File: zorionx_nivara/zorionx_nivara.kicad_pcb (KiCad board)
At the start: 4 copper layers, 102.2 x 83 mm, 29 parts, among them J1 Screw_Terminal_3_P5.00mm, J12 Screw_Terminal_4_P5.00mm, J13 Screw_Terminal_6_P5.00mm, J14 Screw_Terminal_2_P5.00mm, J2 Screw_Terminal_2_P5.00mm, J3 Screw_Terminal_2_P5.00mm, J4 Screw_Terminal_4_P5.00mm, J5 Screw_Terminal_2_P5.00mm, J6 Screw_Terminal_2_P5.00mm, J9 Screw_Terminal_3_P5.00mm, U1 ESP32-S3-WROOM-1, U2 AP63203WU

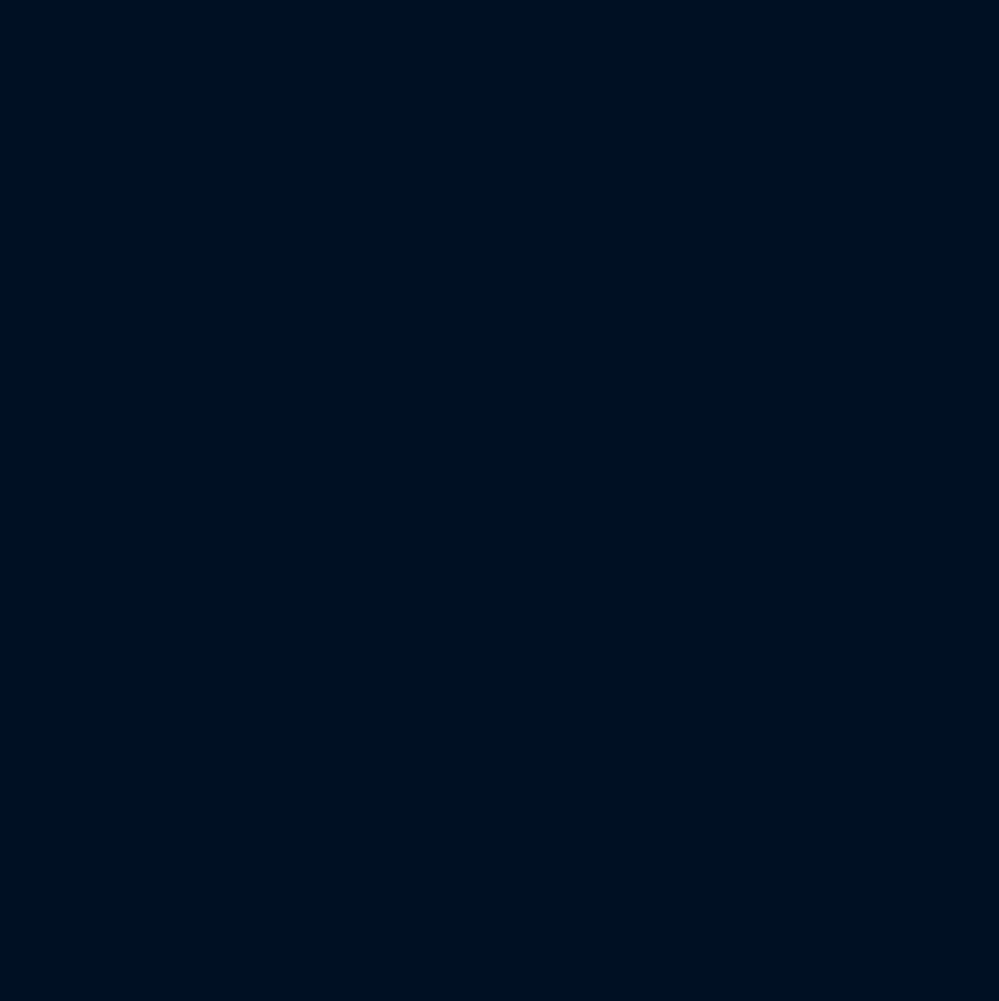
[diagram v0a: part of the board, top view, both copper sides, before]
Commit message: Salvado
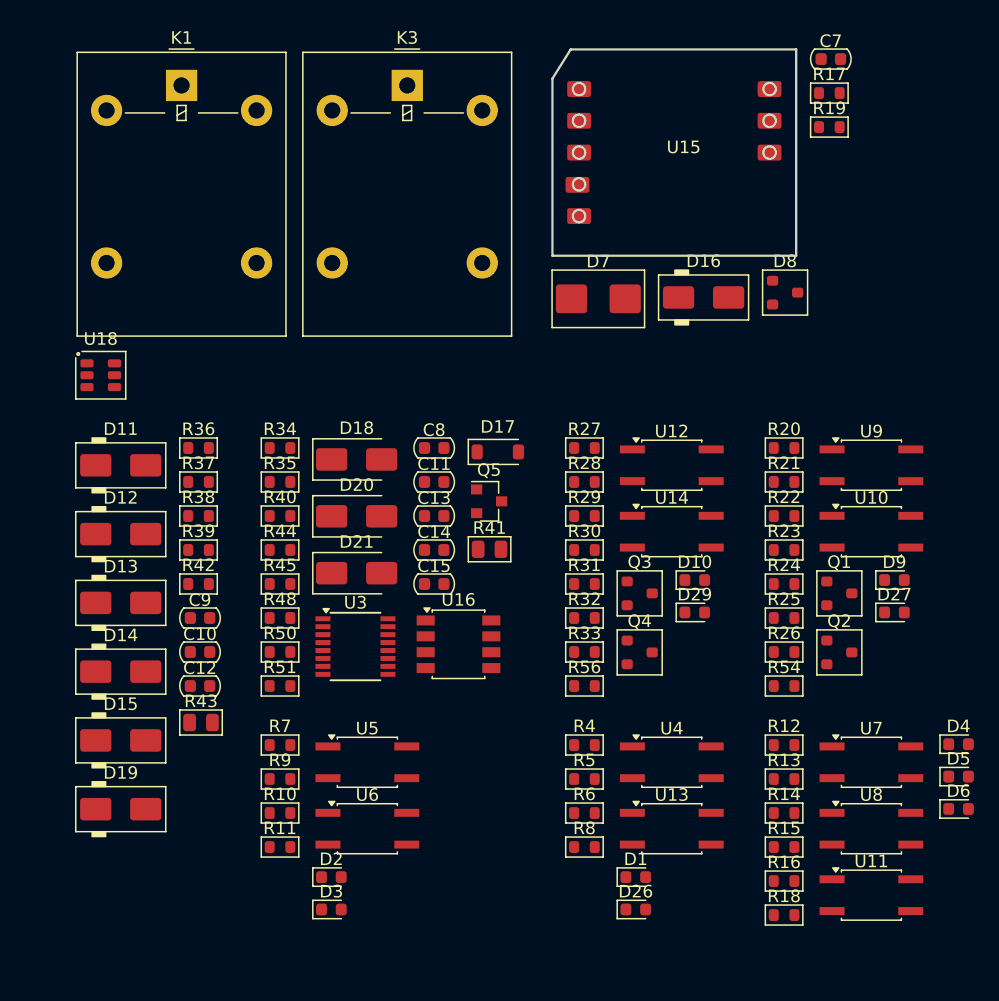
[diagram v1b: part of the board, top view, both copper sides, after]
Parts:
- added C10: 100nF, PCM_Capacitor_SMD_AKL:C_0603_1608Metric, F.Cu at (219.6, 65.1)
- added C11: 0.1uF, PCM_Capacitor_SMD_AKL:C_0603_1608Metric, F.Cu at (238.3, 51.5)
- added C12: 100nF, PCM_Capacitor_SMD_AKL:C_0603_1608Metric, F.Cu at (219.6, 67.9)
- added C13: 220pF, PCM_Capacitor_SMD_AKL:C_0603_1608Metric, F.Cu at (238.3, 54.3)
- added C14: 1uF, PCM_Capacitor_SMD_AKL:C_0603_1608Metric, F.Cu at (238.3, 57.0)
- added C15: 0.1uF, PCM_Capacitor_SMD_AKL:C_0603_1608Metric, F.Cu at (238.3, 59.7)
- added C7: 10uF, PCM_Capacitor_SMD_AKL:C_0603_1608Metric, F.Cu at (270.0, 17.7)
- added C8: 1uF, PCM_Capacitor_SMD_AKL:C_0603_1608Metric, F.Cu at (238.3, 48.8)
- added C9: 100nF, PCM_Capacitor_SMD_AKL:C_0603_1608Metric, F.Cu at (219.6, 62.4)
- added D1: LED ON, LED_SMD:LED_0603_1608Metric, F.Cu at (254.4, 83.1)
- added D10: LED ON, LED_SMD:LED_0603_1608Metric, F.Cu at (259.2, 59.4)
- added D11: SMAJ5.0A, PCM_Diode_SMD_AKL:D_SMA, F.Cu at (213.2, 50.2)
- added D12: SMAJ5.0A, PCM_Diode_SMD_AKL:D_SMA, F.Cu at (213.2, 55.7)
- added D13: SMAJ5.0A, PCM_Diode_SMD_AKL:D_SMA, F.Cu at (213.2, 61.2)
- added D14: SMAJ5.0A, PCM_Diode_SMD_AKL:D_SMA, F.Cu at (213.2, 66.7)
- added D15: SMAJ5.0A, PCM_Diode_SMD_AKL:D_SMA, F.Cu at (213.2, 72.2)
- added D16: SMAJ5.0A, PCM_Diode_SMD_AKL:D_SMA, F.Cu at (259.9, 36.8)
- added D17: BZT52C12_C2891780, Diode_SMD:D_SOD-123, F.Cu at (243.4, 49.1)
- added D18: SMAJ12A, Diode_SMD:D_SMA, F.Cu at (232.1, 49.7)
- added D19: SMAJ5.0A, PCM_Diode_SMD_AKL:D_SMA, F.Cu at (213.2, 77.7)
- added D2: LED ON, LED_SMD:LED_0603_1608Metric, F.Cu at (230.1, 83.1)
- added D20: SMAJ33A, Diode_SMD:D_SMA, F.Cu at (232.1, 54.3)
- added D21: MRA4007T3G, Diode_SMD:D_SMA, F.Cu at (232.1, 58.8)
- added D26: LED ON, LED_SMD:LED_0603_1608Metric, F.Cu at (254.4, 85.7)
- added D27: LED ON, LED_SMD:LED_0603_1608Metric, F.Cu at (275.1, 62.0)
- added D29: LED ON, LED_SMD:LED_0603_1608Metric, F.Cu at (259.2, 62.0)
- added D3: LED ON, LED_SMD:LED_0603_1608Metric, F.Cu at (230.1, 85.7)
- added D4: LED ON, LED_SMD:LED_0603_1608Metric, F.Cu at (280.3, 72.5)
- added D5: LED ON, LED_SMD:LED_0603_1608Metric, F.Cu at (280.3, 75.1)
- added D6: LED ON, LED_SMD:LED_0603_1608Metric, F.Cu at (280.3, 77.7)
- added D7: SMBJ12CA, PCM_Diode_SMD_AKL:D_SMB_TVS, F.Cu at (251.4, 36.9)
- added D8: SM712, PCM_Package_TO_SOT_SMD_AKL:SOT-23, F.Cu at (266.4, 36.4)
- added D9: LED ON, LED_SMD:LED_0603_1608Metric, F.Cu at (275.1, 59.4)
- added K1: G5LE-1, Relay_THT:Relay_SPDT_Omron-G5LE-1, F.Cu at (218.1, 19.8)
- added K3: G5LE-1, Relay_THT:Relay_SPDT_Omron-G5LE-1, F.Cu at (236.2, 19.8)
- added Q1: AO3407A, PCM_Package_TO_SOT_SMD_AKL:SOT-23, F.Cu at (270.7, 60.5)
- added Q2: AO3407A, PCM_Package_TO_SOT_SMD_AKL:SOT-23, F.Cu at (270.7, 65.2)
- added Q3: IRLML0040, PCM_Package_TO_SOT_SMD_AKL:SOT-23, F.Cu at (254.7, 60.5)
- added Q4: IRLML0040, PCM_Package_TO_SOT_SMD_AKL:SOT-23, F.Cu at (254.7, 65.2)
- added Q5: IRLML6402TRPBF-JSM, PCM_4ms_Package_SOT:SOT-23, F.Cu at (242.7, 53.1)
- added R10: 1k, PCM_Resistor_SMD_AKL:R_0603_1608Metric, F.Cu at (226.0, 78.0)
- added R11: 1k, PCM_Resistor_SMD_AKL:R_0603_1608Metric, F.Cu at (226.0, 80.7)
- added R12: 180, PCM_Resistor_SMD_AKL:R_0603_1608Metric, F.Cu at (266.3, 72.6)
- added R13: 180, PCM_Resistor_SMD_AKL:R_0603_1608Metric, F.Cu at (266.3, 75.3)
- added R14: 1k, PCM_Resistor_SMD_AKL:R_0603_1608Metric, F.Cu at (266.3, 78.0)
- added R15: 180, PCM_Resistor_SMD_AKL:R_0603_1608Metric, F.Cu at (266.3, 80.7)
- added R16: 1k, PCM_Resistor_SMD_AKL:R_0603_1608Metric, F.Cu at (266.3, 83.5)
- added R17: R_0603, PCM_Resistor_SMD_AKL:R_0603_1608Metric, F.Cu at (269.9, 20.4)
- added R18: 1k, PCM_Resistor_SMD_AKL:R_0603_1608Metric, F.Cu at (266.3, 86.2)
- added R19: R_0603, PCM_Resistor_SMD_AKL:R_0603_1608Metric, F.Cu at (269.9, 23.2)
- added R20: 100, PCM_Resistor_SMD_AKL:R_0603_1608Metric, F.Cu at (266.3, 48.8)
- added R21: 100, PCM_Resistor_SMD_AKL:R_0603_1608Metric, F.Cu at (266.3, 51.5)
- added R22: 100k, PCM_Resistor_SMD_AKL:R_0603_1608Metric, F.Cu at (266.3, 54.3)
- added R23: 100, PCM_Resistor_SMD_AKL:R_0603_1608Metric, F.Cu at (266.3, 57.0)
- added R24: 100k, PCM_Resistor_SMD_AKL:R_0603_1608Metric, F.Cu at (266.3, 59.7)
- added R25: 100, PCM_Resistor_SMD_AKL:R_0603_1608Metric, F.Cu at (266.3, 62.4)
- added R26: 1.5k, PCM_Resistor_SMD_AKL:R_0603_1608Metric, F.Cu at (266.3, 65.1)
- added R27: 100, PCM_Resistor_SMD_AKL:R_0603_1608Metric, F.Cu at (250.3, 48.8)
- added R28: 30k, PCM_Resistor_SMD_AKL:R_0603_1608Metric, F.Cu at (250.3, 51.5)
- added R29: 22k, PCM_Resistor_SMD_AKL:R_0603_1608Metric, F.Cu at (250.3, 54.3)
- added R30: 100, PCM_Resistor_SMD_AKL:R_0603_1608Metric, F.Cu at (250.3, 57.0)
- added R31: 30K, PCM_Resistor_SMD_AKL:R_0603_1608Metric, F.Cu at (250.3, 59.7)
- added R32: 22K, PCM_Resistor_SMD_AKL:R_0603_1608Metric, F.Cu at (250.3, 62.4)
- added R33: 1.7K, PCM_Resistor_SMD_AKL:R_0603_1608Metric, F.Cu at (250.3, 65.1)
- added R34: 4.7K, PCM_Resistor_SMD_AKL:R_0603_1608Metric, F.Cu at (226.0, 48.8)
- added R35: 4.7K, PCM_Resistor_SMD_AKL:R_0603_1608Metric, F.Cu at (226.0, 51.5)
- added R36: 100K, PCM_Resistor_SMD_AKL:R_0603_1608Metric, F.Cu at (219.5, 48.8)
- added R37: 10K, PCM_Resistor_SMD_AKL:R_0603_1608Metric, F.Cu at (219.5, 51.5)
- added R38: 25K, PCM_Resistor_SMD_AKL:R_0603_1608Metric, F.Cu at (219.5, 54.3)
- added R39: 10K, PCM_Resistor_SMD_AKL:R_0603_1608Metric, F.Cu at (219.5, 57.0)
- added R4: 180, PCM_Resistor_SMD_AKL:R_0603_1608Metric, F.Cu at (250.3, 72.6)
- added R40: 100K, PCM_Resistor_SMD_AKL:R_0603_1608Metric, F.Cu at (226.0, 54.3)
- added R41: 15, PCM_Resistor_SMD_AKL:R_0805_2012Metric, F.Cu at (242.7, 56.9)
- added R42: 1k, PCM_Resistor_SMD_AKL:R_0603_1608Metric, F.Cu at (219.5, 59.7)
- added R43: 145, PCM_Resistor_SMD_AKL:R_0805_2012Metric, F.Cu at (219.7, 70.8)
- added R44: 4.7K, PCM_Resistor_SMD_AKL:R_0603_1608Metric, F.Cu at (226.0, 57.0)
- added R45: 4.7K, PCM_Resistor_SMD_AKL:R_0603_1608Metric, F.Cu at (226.0, 59.7)
- added R48: 10K, PCM_Resistor_SMD_AKL:R_0603_1608Metric, F.Cu at (226.0, 62.4)
- added R5: 180, PCM_Resistor_SMD_AKL:R_0603_1608Metric, F.Cu at (250.3, 75.3)
- added R50: 0, PCM_Resistor_SMD_AKL:R_0603_1608Metric, F.Cu at (226.0, 65.1)
- added R51: 2.5K, PCM_Resistor_SMD_AKL:R_0603_1608Metric, F.Cu at (226.0, 67.9)
- added R54: 1.5k, PCM_Resistor_SMD_AKL:R_0603_1608Metric, F.Cu at (266.3, 67.9)
- added R56: 1.7K, PCM_Resistor_SMD_AKL:R_0603_1608Metric, F.Cu at (250.3, 67.9)
- added R6: 1k, PCM_Resistor_SMD_AKL:R_0603_1608Metric, F.Cu at (250.3, 78.0)
- added R7: 180, PCM_Resistor_SMD_AKL:R_0603_1608Metric, F.Cu at (226.0, 72.6)
- added R8: 1k, PCM_Resistor_SMD_AKL:R_0603_1608Metric, F.Cu at (250.3, 80.7)
- added R9: 180, PCM_Resistor_SMD_AKL:R_0603_1608Metric, F.Cu at (226.0, 75.3)
- added U10: LTV-357T, Package_SO:SO-4_4.4x3.6mm_P2.54mm, F.Cu at (273.3, 55.5)
- added U11: LTV-357T, Package_SO:SO-4_4.4x3.6mm_P2.54mm, F.Cu at (273.3, 84.6)
- added U12: LTV-357T, Package_SO:SO-4_4.4x3.6mm_P2.54mm, F.Cu at (257.3, 50.2)
- added U13: LTV-357T, Package_SO:SO-4_4.4x3.6mm_P2.54mm, F.Cu at (257.3, 79.3)
- added U14: LTV-357T, Package_SO:SO-4_4.4x3.6mm_P2.54mm, F.Cu at (257.3, 55.5)
- added U15: ~, Biblioteca_BryanFernandez_Huellas:YLPTEC RSM3485ECHT, F.Cu at (258.3, 25.3)
- added U16: GP8201S-TC50-EW, Package_SO:SSOP-8_3.95x5.21x3.27mm_P1.27mm, F.Cu at (240.3, 64.5)
- added U18: LANKE LK1802, PCM_Package_TO_SOT_SMD_AKL:SOT-23-6, F.Cu at (211.6, 43.0)
- added U3: GP8303-TC50-EW, Package_SO:SSOP-16_3.9x4.9mm_P0.635mm, F.Cu at (232.0, 64.7)
- added U4: LTV-357T, Package_SO:SO-4_4.4x3.6mm_P2.54mm, F.Cu at (257.3, 74.0)
- added U5: LTV-357T, Package_SO:SO-4_4.4x3.6mm_P2.54mm, F.Cu at (233.0, 74.0)
- added U6: LTV-357T, Package_SO:SO-4_4.4x3.6mm_P2.54mm, F.Cu at (233.0, 79.3)
- added U7: LTV-357T, Package_SO:SO-4_4.4x3.6mm_P2.54mm, F.Cu at (273.3, 74.0)
- added U8: LTV-357T, Package_SO:SO-4_4.4x3.6mm_P2.54mm, F.Cu at (273.3, 79.3)
- added U9: LTV-357T, Package_SO:SO-4_4.4x3.6mm_P2.54mm, F.Cu at (273.3, 50.2)
- L1: value L_Iron -> 6.8uH
- R1: value 22K -> 196K
- R2: value 22K -> ~
- R3: value 22K -> 62K
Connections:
- net /board_zorionx-nivara/D_IN1 renamed /D_IN1
- net /board_zorionx-nivara/D_IN2 renamed /D_IN2
- net /board_zorionx-nivara/PowerSupply/sw renamed /board_zorionx-nivara/PowerSupply +3V/sw
- net /board_zorionx-nivara/PowerSupply/vout renamed /board_zorionx-nivara/PowerSupply +3V/vout
- H1 pad 1: unconnected-(H1-Pad1) -> GND
- H2 pad 1: unconnected-(H2-Pad1) -> GND
- U1 pad 10: unconnected-(U1-IO17-Pad10) -> /board_zorionx-nivara/Driver_RS485/UART_IN
- U1 pad 11: unconnected-(U1-IO18-Pad11) -> /board_zorionx-nivara/Driver_RS485/UART_OUT
- U1 pad 12: unconnected-(U1-IO8-Pad12) -> /board_zorionx-nivara/DIGITAL_IN/ESP32-S3_DIGITAL_IN_1
- U1 pad 15: unconnected-(U1-IO3-Pad15) -> /board_zorionx-nivara/ANALOG_IN/ESP32-S3_4-20_IN
- U1 pad 17: unconnected-(U1-IO9-Pad17) -> /board_zorionx-nivara/DIGITAL_IN/ESP32-S3_DIGITAL_IN_2
- U1 pad 18: unconnected-(U1-IO10-Pad18) -> /board_zorionx-nivara/DIGITAL_IN/ESP32-S3_RUN_IN
- U1 pad 19: unconnected-(U1-IO11-Pad19) -> /board_zorionx-nivara/RELAY_#1_#2/ESP32-S3_RY1
- U1 pad 20: unconnected-(U1-IO12-Pad20) -> /board_zorionx-nivara/RELAY_#1_#2/ESP32-S3_RLY2
- U1 pad 21: unconnected-(U1-IO13-Pad21) -> /board_zorionx-nivara/Output_PNP/ESP32-S3_PNP_OUT_2
- U1 pad 22: unconnected-(U1-IO14-Pad22) -> /board_zorionx-nivara/Output_PNP/ESP32-S3_PNP_OUT_1
- U1 pad 27: unconnected-(U1-IO0-Pad27) -> /board_zorionx-nivara/INPUTS_NPN/ESP32-S3_NPN_IN_1
- U1 pad 32: unconnected-(U1-IO39-Pad32) -> /board_zorionx-nivara/Output_NPN/ESP32-S3_NPN_OUT_1
- U1 pad 33: unconnected-(U1-IO40-Pad33) -> /board_zorionx-nivara/Output_NPN/ESP32-S3_NPN_OUT_2
- U1 pad 36: /board_zorionx-nivara/Driver_RS485/UART_OUT -> unconnected-(U1-RXD0-Pad36)
- U1 pad 37: /board_zorionx-nivara/Driver_RS485/UART_IN -> unconnected-(U1-TXD0-Pad37)
- U1 pad 38: unconnected-(U1-IO2-Pad38) -> /board_zorionx-nivara/ANALOG_IN/ESP32-S3_A0_32_IN_1
- U1 pad 39: unconnected-(U1-IO1-Pad39) -> /board_zorionx-nivara/ANALOG_IN/ESP32-S3_A0_10_IN_1
- U1 pad 4: unconnected-(U1-IO4-Pad4) -> /board_zorionx-nivara/INPUTS_NPN/ESP32-S3_NPN_IN_2
- U1 pad 5: unconnected-(U1-IO5-Pad5) -> /board_zorionx-nivara/INPUTS_PNP/ESP32-S3_PNP_IN_1
- U1 pad 6: unconnected-(U1-IO6-Pad6) -> /board_zorionx-nivara/INPUTS_PNP/ESP32-S3_PNP_IN_2
- U1 pad 7: unconnected-(U1-IO7-Pad7) -> /board_zorionx-nivara/ANALOG_OUT/ESP32-S3_SEL_VOUT
- U1 pad 8: unconnected-(U1-IO15-Pad8) -> /board_zorionx-nivara/ANALOG_OUT/SDA_V
- U1 pad 9: unconnected-(U1-IO16-Pad9) -> /board_zorionx-nivara/ANALOG_OUT/SCLK_V
